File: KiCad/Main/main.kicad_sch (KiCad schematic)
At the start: 9 parts, among them U1 ESP32-S3-DEVKITC-1-N8R2

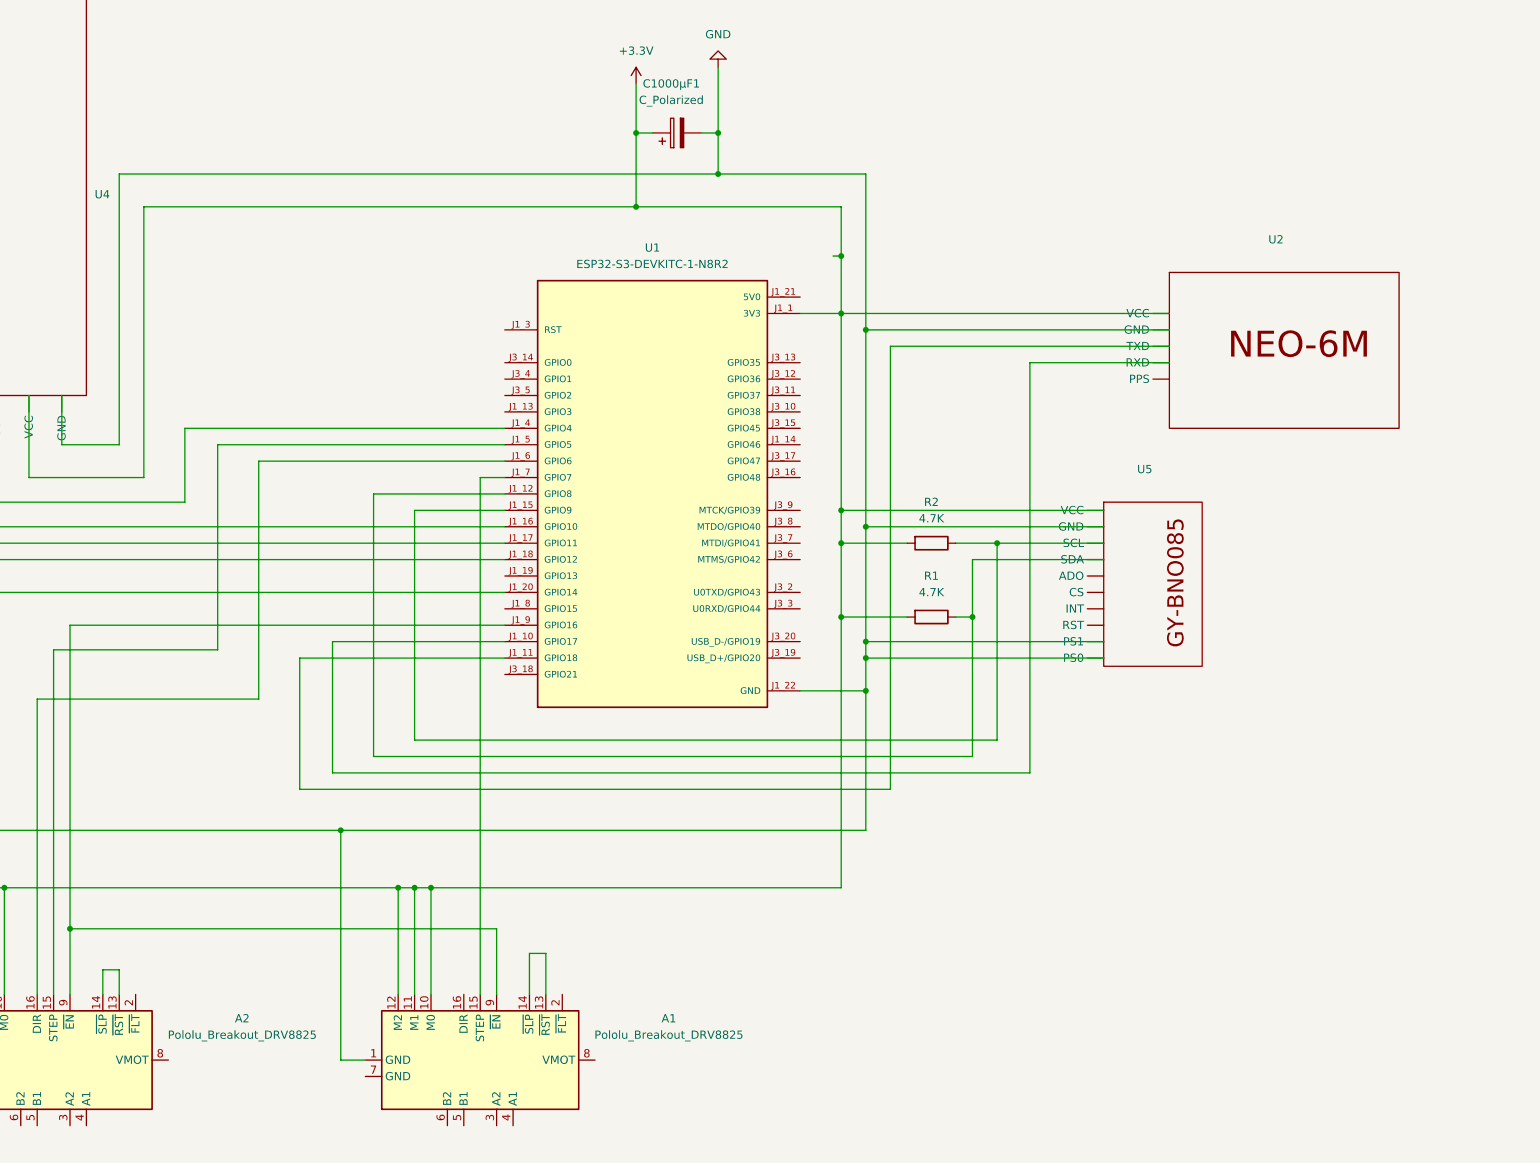
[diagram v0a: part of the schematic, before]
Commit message: partiel
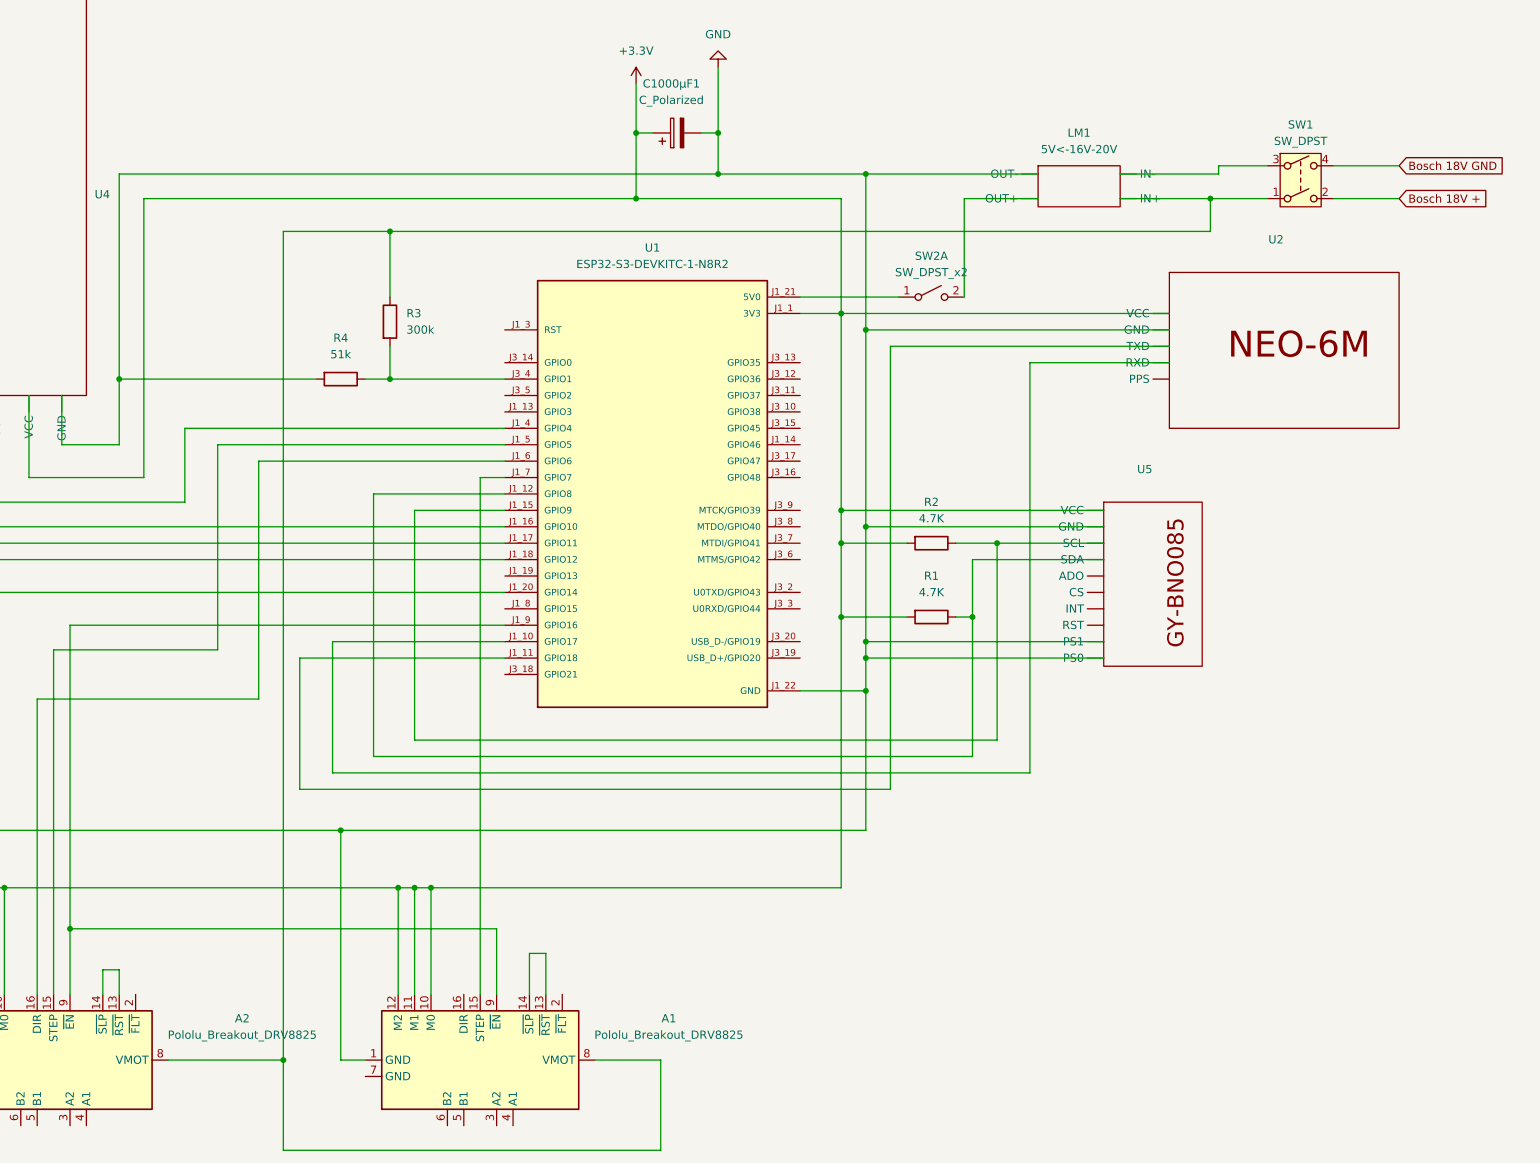
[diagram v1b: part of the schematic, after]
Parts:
- added LM1: 5V<-16V-20V, symbol GH:LM2596_DC-DC
- added R3: 300k, symbol Device:R
- added R4: 51k, symbol Device:R
- added SW1: SW_DPST, symbol Switch:SW_DPST
- added SW2: SW_DPST_x2, symbol Switch:SW_DPST_x2
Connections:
- net GND: now also LM1. (IN+), R4.2
- net at A1.8 (VMOT): now also A2.8 (VMOT), LM1. (IN+), R3.1, SW1.1
- net at U1.J1_21 (5V0): now also SW2.1 (A)
- net at U1.J3_4 (GPIO1): now also R3.2, R4.1
- new net: LM1. (IN+), SW1.3
- new net: LM1. (IN+), SW2.2 (B)
- new net Bosch 18V +: SW1.2
- new net Bosch 18V GND: SW1.4

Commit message: ok
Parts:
- removed A1, A2: Pololu_Breakout_DRV8825, Module:Pololu_Breakout-16_15.2x20.3mm, symbol Driver_Motor:Pololu_Breakout_DRV8825
- removed C1000µF1: C_Polarized, symbol Device:C_Polarized
- removed LM1: 5V<-16V-20V, symbol GH:LM2596_DC-DC
- removed R1, R2: 4.7K, symbol Device:R
- removed R3: 300k, symbol Device:R
- removed R4: 51k, symbol Device:R
- removed SW1: SW_DPST, symbol Switch:SW_DPST
- removed U5: ~, symbol gy-bno08x:gy-bno08x
- added J2: Conn_01x10_Pin, symbol Connector:Conn_01x10_Pin
- added J5, J6: Conn_01x02_Pin, symbol Connector:Conn_01x02_Pin
- added J8: RJ45, symbol Connector:RJ45
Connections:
- net GND: now also J5.1 (Pin_1), J6.1 (Pin_1), J8.7
- net at SW2.2 (B): now also U1.J1_21 (5V0)
- net at U1.J1_12 (GPIO8): now also J8.5
- net ALT/STEP: now reaches U1.J1_7 (GPIO7)
- net ALT/STEP: now also J2.9 (Pin_9)
- net EN: now reaches U1.J1_9 (GPIO16)
- net EN: now also J2.6 (Pin_6)
- net at SW2.1 (A): now also J5.2 (Pin_2), J6.2 (Pin_2); no longer U1.J1_21 (5V0)
- net AZ/STEP: now reaches U1.J1_5 (GPIO5)
- net AZ/STEP: now also J2.7 (Pin_7)
- net AZ/DIR: now reaches U1.J1_6 (GPIO6)
- net AZ/DIR: now also J2.8 (Pin_8)
- net at U1.J1_15 (GPIO9): now also J8.6
- net RST/SLP: now reaches U1.J1_13 (GPIO3)
- net RST/SLP: now also J2.5 (Pin_5)
- net ALT/DIR: now reaches U1.J1_8 (GPIO15)
- net ALT/DIR: now also J2.10 (Pin_10)
- net at U1.J3_4 (GPIO1): now also J2.1 (Pin_1)
- net M0: now reaches U1.J3_5 (GPIO2)
- net M0: now also J2.2 (Pin_2)
- net M2: now reaches U1.J3_6 (MTMS/GPIO42)
- net M2: now also J2.4 (Pin_4)
- net M1: now reaches U1.J3_7 (MTDI/GPIO41)
- net M1: now also J2.3 (Pin_3)
- net +3.3V renamed 3V3
- net 3V3: now also J8.8
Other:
- added sheet Alimentation (Alimentation.kicad_sch)
- added sheet BNO085 (bno085.kicad_sch)
- added sheet Moteur et alimentation (AlimentationBis.kicad_sch)
- moved on the sheet: SW2A, U2

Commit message: ok
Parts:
- removed U1: ESP32-S3-DEVKITC-1-N8R2, ESP32-S3-DEVKITC-1-N8R2:XCVR_ESP32-S3-DEVKITC-1-N8R2, symbol ESP32-S3-DEVKITC-1-N8R2:ESP32-S3-DEVKITC-1-N8R2
- removed U2: ~, symbol neo-6M:NEO-6M
- removed U4: ~, symbol GMT020-02:GMT020-02
- added C1000µF2: C_Polarized, Capacitor_THT:CP_Radial_D17.0mm_P7.50mm, symbol Device:C_Polarized
- added J1: Vers GPS, Connector_JST:JST_EH_B5B-EH-A_1x05_P2.50mm_Vertical, symbol Connector:Conn_01x05_Pin
- added J3: Vers Display, Connector_JST:JST_EH_B7B-EH-A_1x07_P2.50mm_Vertical, symbol Connector:Conn_01x07_Pin
- added U5: ESP32-S3-DevKitC, PCM_Espressif:ESP32-S3-DevKitC, symbol PCM_Espressif:ESP32-S3-DevKitC
- J2: value Conn_01x10_Pin -> Vers Moteurs; footprint (none) -> Connector_JST:JST_EH_B10B-EH-A_1x10_P2.50mm_Vertical
- J5, J6: footprint (none) -> Connector_JST:JST_EH_B2B-EH-A_1x02_P2.50mm_Vertical
- J8: footprint (none) -> Connector_RJ:RJ45_Amphenol_54602-x08_Horizontal
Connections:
- net ALT/DIR: now also U5.8 (GPIO15/ADC2_CH4/32K_P)
- net ALT/STEP: now also U5.7 (GPIO7/ADC1_CH6)
- net AZ/DIR: now also U5.6 (GPIO6/ADC1_CH5)
- net AZ/STEP: now also U5.5 (GPIO5/ADC1_CH4)
- net EN: now also U5.9 (GPIO16/ADC2_CH5/32K_N)
- net GND: now also C1000µF2.2, J1.2 (Pin_2), J3.7 (Pin_7), U5.22 (GND), U5.23 (GND), U5.24 (GND), U5.44 (GND)
- net M0: now also U5.40 (GPIO2/ADC1_CH1)
- net M1: now also U5.38 (GPIO41/MTDI)
- net M2: now also U5.39 (GPIO42/MTMS)
- net RST/SLP: now also U5.13 (GPIO3/ADC1_CH2)
- net PontDiviseur: now reaches J2.1 (Pin_1)
- net PontDiviseur: now also U5.41 (GPIO1/ADC1_CH0)
- net SDA: now reaches J8.5
- net SDA: now also U5.12 (GPIO8/ADC1_CH7)
- net SCL: now reaches J8.6
- net SCL: now also U5.15 (GPIO9/ADC1_CH8)
- net at SW2.2 (B): now also C1000µF2.1, U5.21 (5V)
- net 3V3 renamed VCC
- net VCC: now also J1.1 (Pin_1), J3.6 (Pin_6), U5.1 (3V3), U5.2 (3V3)
- new net CS: J3.1 (Pin_1), U5.16 (GPIO10/ADC1_CH9)
- new net DC: J3.2 (Pin_2), U5.4 (GPIO4/ADC1_CH3)
- new net RST: J3.3 (Pin_3), U5.20 (GPIO14/ADC2_CH3)
- new net RXD: J1.4 (Pin_4), U5.10 (GPIO17/ADC2_CH6)
- new net SCL_DSP: J3.5 (Pin_5), U5.18 (GPIO12/ADC2_CH1)
- new net SDA_DSP: J3.4 (Pin_4), U5.17 (GPIO11/ADC2_CH0)
- new net TXD: J1.3 (Pin_3), U5.11 (GPIO18/ADC2_CH7)
- no-connect marks 0 -> 1
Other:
- sheet Moteur et alimentation renamed Moteurs et alimentation
- removed sheet Alimentation
- added sheet GMT020-02 (display.kicad_sch)
- added sheet NEO-6M (GPS.kicad_sch)
- sheet Moteurs et alimentation: file AlimentationBis.kicad_sch -> Moteurs et alimentation.kicad_sch
- moved on the sheet: J2, J5, J6, J8, SW2A

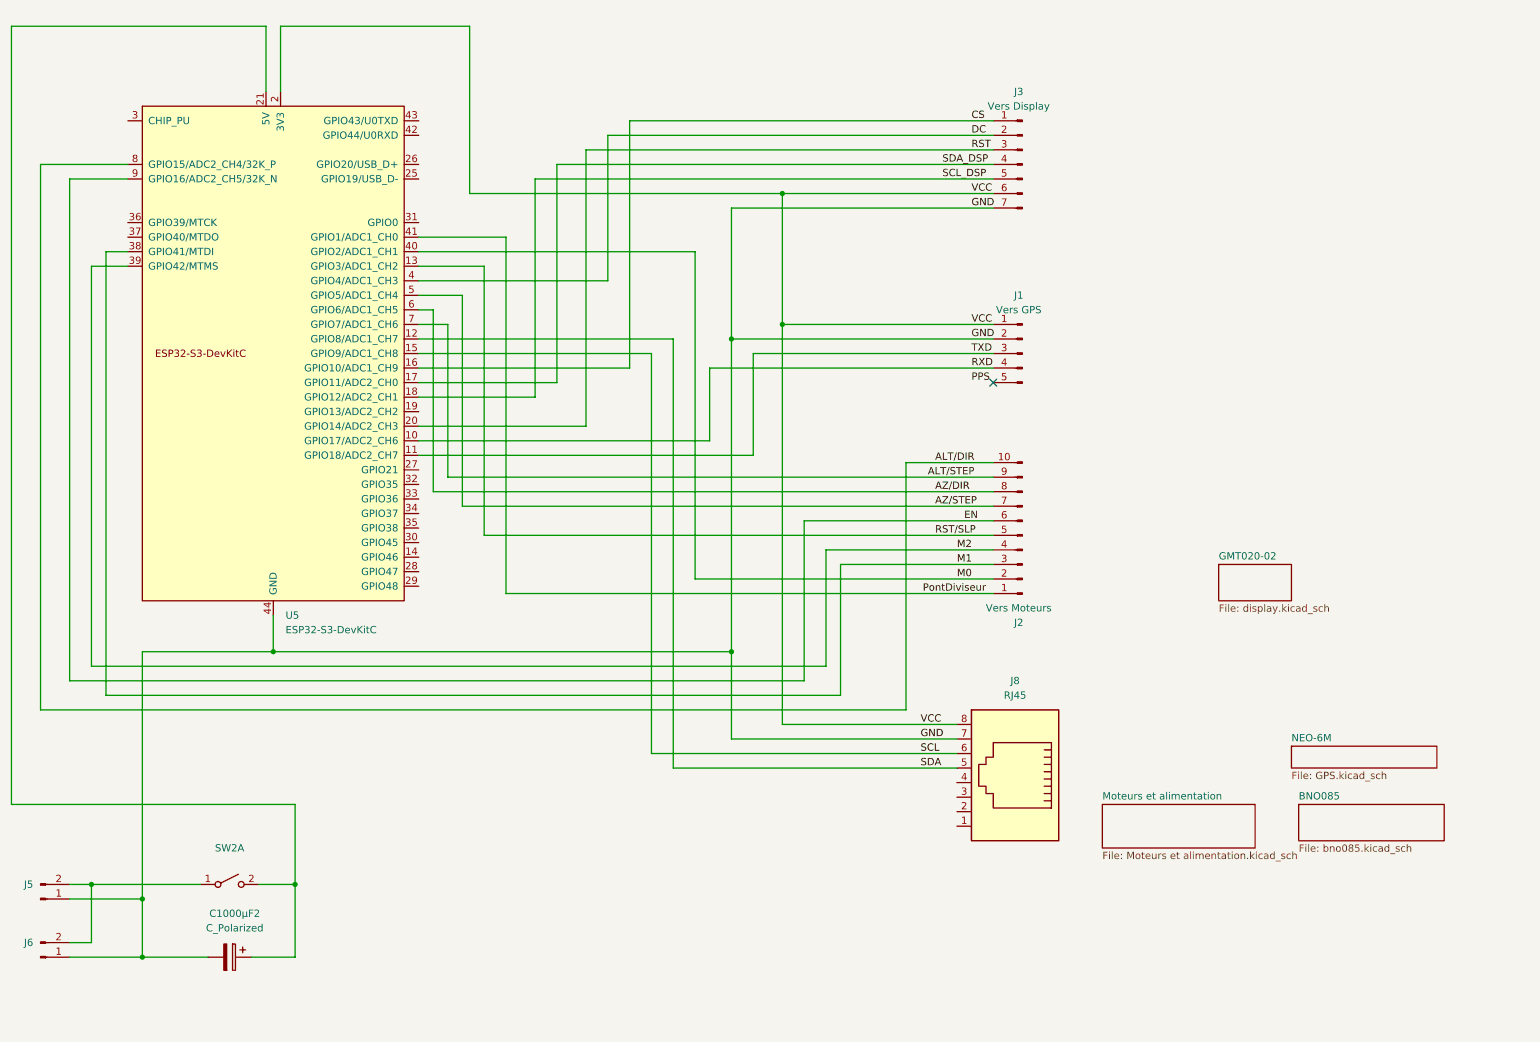
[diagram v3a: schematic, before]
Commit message: ok
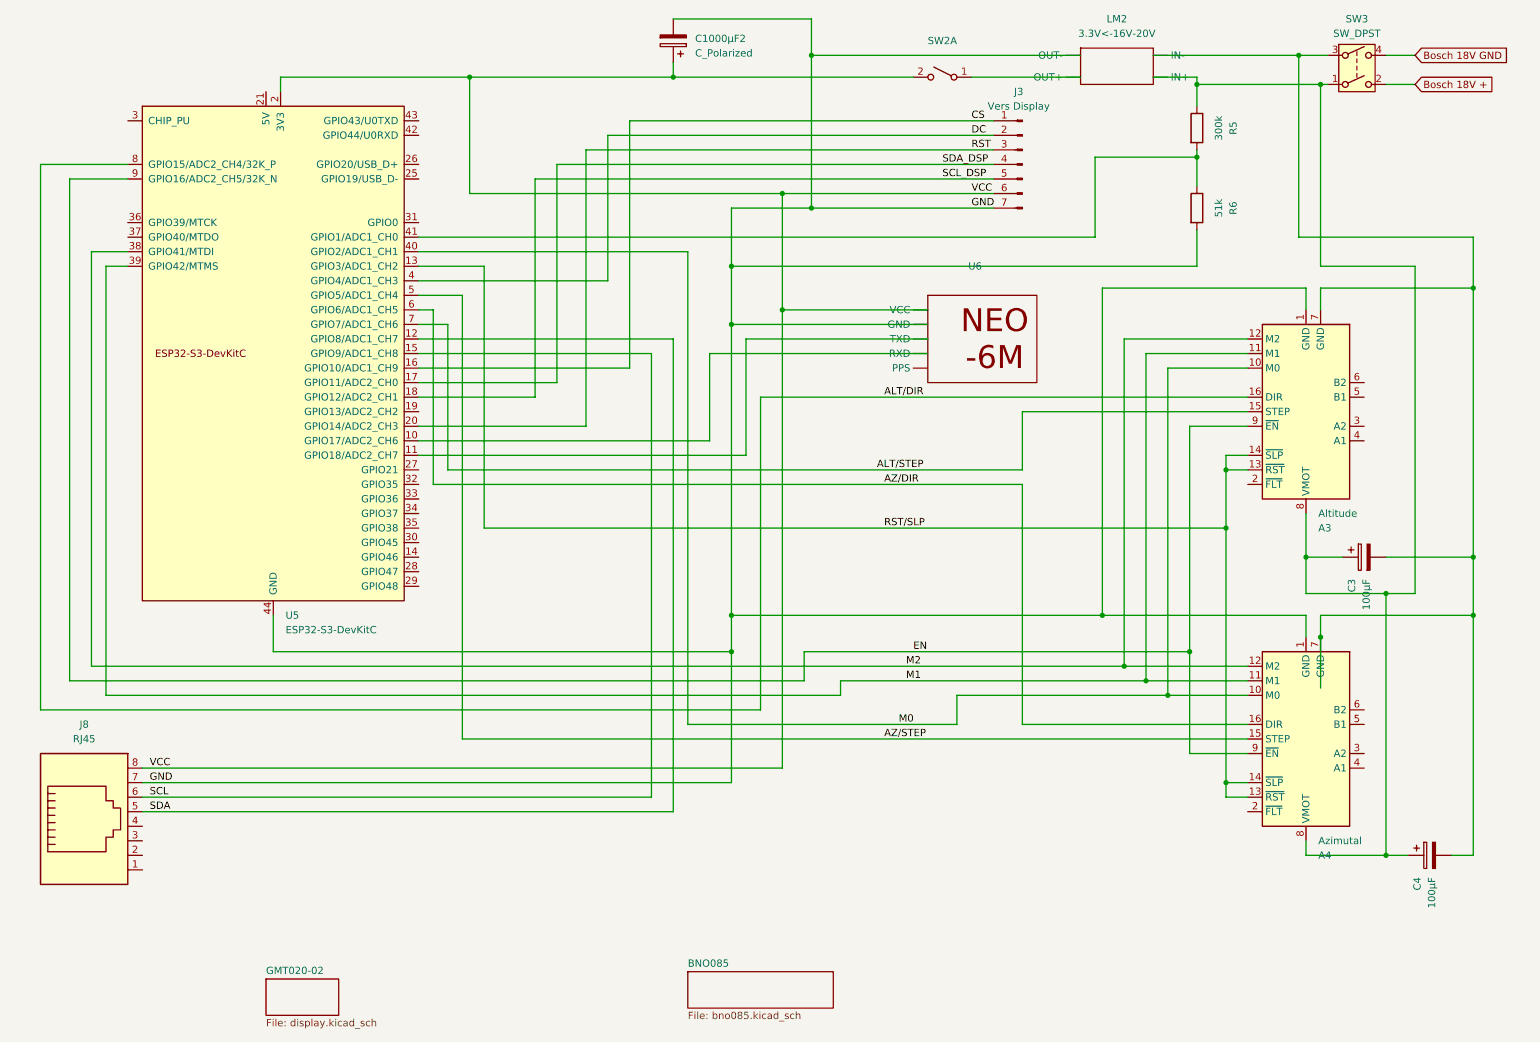
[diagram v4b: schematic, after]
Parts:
- removed J1: Vers GPS, Connector_JST:JST_EH_B5B-EH-A_1x05_P2.50mm_Vertical, symbol Connector:Conn_01x05_Pin
- removed J2: Vers Moteurs, Connector_JST:JST_EH_B10B-EH-A_1x10_P2.50mm_Vertical, symbol Connector:Conn_01x10_Pin
- removed J5, J6: Conn_01x02_Pin, Connector_JST:JST_EH_B2B-EH-A_1x02_P2.50mm_Vertical, symbol Connector:Conn_01x02_Pin
- added A3: Altitude, Module:Pololu_Breakout-16_15.2x20.3mm, symbol Driver_Motor:Pololu_Breakout_DRV8825
- added A4: Azimutal, Module:Pololu_Breakout-16_15.2x20.3mm, symbol Driver_Motor:Pololu_Breakout_DRV8825
- added C3, C4: 100µF, PCM_Capacitor_THT_AKL:CP_Radial_D8.0mm_P5.00mm, symbol PCM_Capacitor_AKL:CP_Radial_D8.0mm_P5.00mm
- added LM2: 3.3V<-16V-20V, symbol GH:LM2596_DC-DC
- added R5: 300k, symbol Device:R
- added R6: 51k, symbol Device:R
- added SW3: SW_DPST, symbol Switch:SW_DPST
- added U6: ~, symbol GH:NEO-6M
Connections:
- net ALT/DIR: now also A3.16 (DIR)
- net ALT/STEP: now also A3.15 (STEP)
- net AZ/DIR: now also A4.16 (DIR)
- net AZ/STEP: now also A4.15 (STEP)
- net EN: now also A3.9 (~{EN}), A4.9 (~{EN})
- net GND: now also A3.1 (GND), A4.1 (GND), LM2. (IN+), R6.2, U6. (PPS)
- net M0: now also A3.10 (M0), A4.10 (M0)
- net M1: now also U5.39 (GPIO42/MTMS), A3.11 (M1), A4.11 (M1); no longer U5.38 (GPIO41/MTDI)
- net M2: now also U5.38 (GPIO41/MTDI), A3.12 (M2), A4.12 (M2); no longer U5.39 (GPIO42/MTMS)
- net RST/SLP: now also A3.13 (~{RST}), A3.14 (~{SLP}), A4.13 (~{RST}), A4.14 (~{SLP})
- net VCC: now also C1000µF2.1, SW2.2 (B), U6. (PPS)
- net at SW2.1 (A): now also LM2. (IN+)
- net PontDiviseur: no longer names the net of U5.41 (GPIO1/ADC1_CH0)
- net PontDiviseur: now also R5.2, R6.1
- net RXD: no longer names the net of U5.10 (GPIO17/ADC2_CH6)
- net RXD: now also U6. (PPS)
- net TXD: no longer names the net of U5.11 (GPIO18/ADC2_CH7)
- net TXD: now also U6. (PPS)
- new net: A3.7 (GND), A4.7 (GND), C3.2, C4.2, LM2. (IN+), SW3.3
- new net: A3.8 (VMOT), A4.8 (VMOT), C3.1, C4.1, LM2. (IN+), R5.1, SW3.1
- new net Bosch 18V +: SW3.2
- new net Bosch 18V GND: SW3.4
- now unconnected: U5.21 (5V)
- no-connect marks 1 -> 0
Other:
- removed sheet Moteurs et alimentation
- removed sheet NEO-6M
- moved on the sheet: C1000µF2, J8, SW2A
